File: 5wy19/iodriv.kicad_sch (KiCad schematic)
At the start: 17 parts, among them IC10 MC33385, IC3 74HCT574, IC4 HIP0045, IC6 MC33385, IC8 MC33385, Q7 BCR183

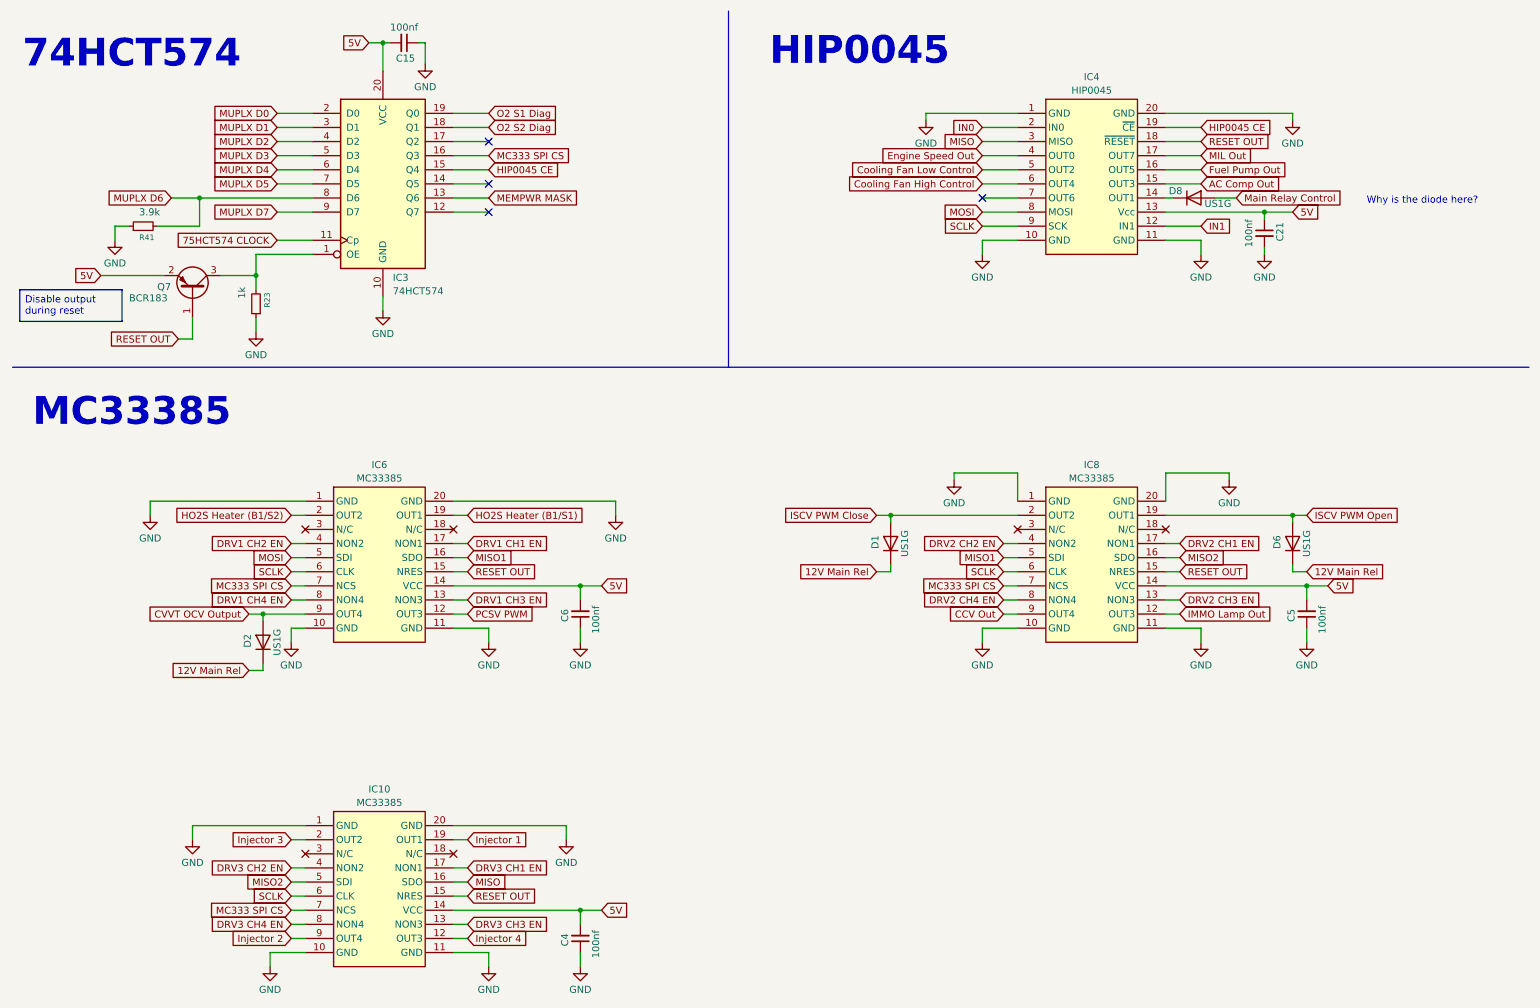
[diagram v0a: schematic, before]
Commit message: Final schematic (except maybe some oversights)
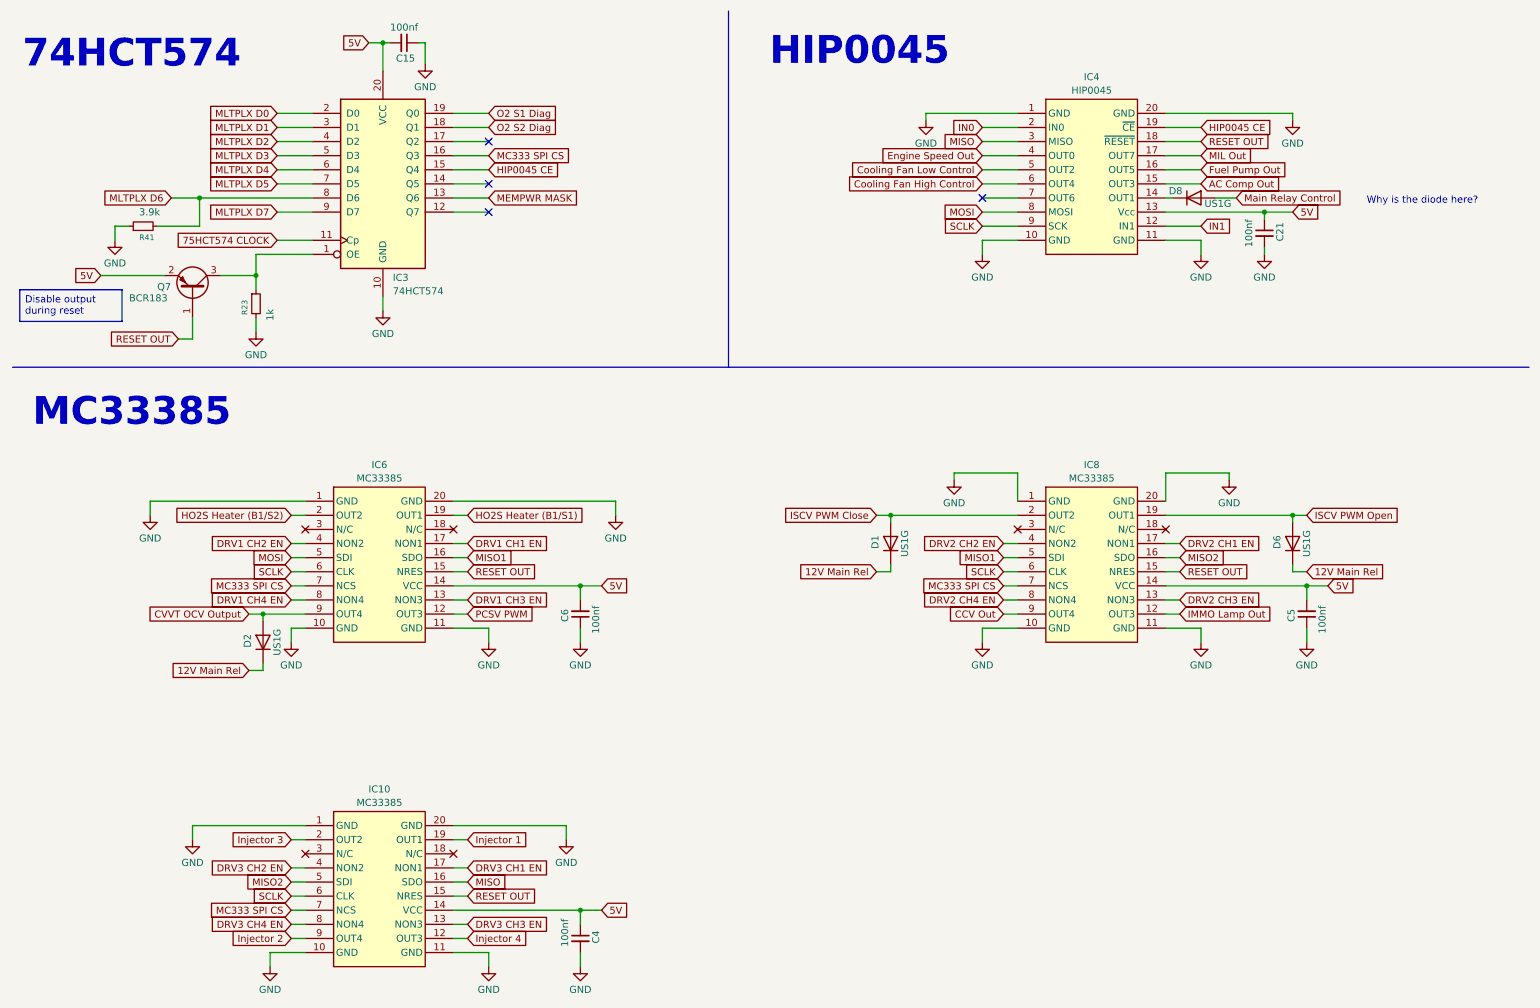
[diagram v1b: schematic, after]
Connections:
- net 5V: now also C4.1; no longer C4.2
- net GND: now also C4.2, R23.2; no longer C4.1, R23.1
- net at IC3.1 (OE), Q7.3 (C): now also R23.1; no longer R23.2
- net MUPLX D0 renamed MLTPLX D0
- net MUPLX D1 renamed MLTPLX D1
- net MUPLX D2 renamed MLTPLX D2
- net MUPLX D3 renamed MLTPLX D3
- net MUPLX D4 renamed MLTPLX D4
- net MUPLX D5 renamed MLTPLX D5
- net MUPLX D6 renamed MLTPLX D6
- net MUPLX D7 renamed MLTPLX D7
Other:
- moved on the sheet: C4, R23
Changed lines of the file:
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@@
 		)
 	)
-	(global_label "MUPLX D0"
-		(shape input)
-		(at 59.69 30.48 180)
-		(fields_autoplaced yes)
-		(effects
-			(font
-				(size 1.27 1.27)
-			)
-			(justify right)
-		)
-		(property "Intersheetrefs" "${INTERSHEET_REFS}"
-			(at 46.9682 30.48 0)
-			(effects
-				(font
-					(size 1.27 1.27)
-				)
-				(justify right)
-				(hide yes)
-			)
-		)
-	)
 	(global_label "Injector 4"
 		(shape input)
@@
 		)
 	)
-	(global_label "MUPLX D4"
-		(shape input)
-		(at 59.69 40.64 180)
-		(fields_autoplaced yes)
-		(effects
-			(font
-				(size 1.27 1.27)
-			)
-			(justify right)
-		)
-		(property "Intersheetrefs" "${INTERSHEET_REFS}"
-			(at 46.9682 40.64 0)
-			(effects
-				(font
-					(size 1.27 1.27)
-				)
-				(justify right)
-				(hide yes)
-			)
-		)
-	)
 	(global_label "DRV3 CH1 EN"
 		(shape input)
@@
 		)
 	)
-	(global_label "MUPLX D6"
+	(global_label "5V"
 		(shape input)
-		(at 40.64 45.72 180)
+		(at 27.94 59.69 180)
 		(fields_autoplaced yes)
 		(effects
@@
 		)
 		(property "Intersheetrefs" "${INTERSHEET_REFS}"
-			(at 27.9182 45.72 0)
+			(at 22.6567 59.69 0)
 			(effects
 				(font
@@
 		)
 	)
-	(global_label "5V"
+	(global_label "MLTPLX D5"
 		(shape input)
-		(at 27.94 59.69 180)
+		(at 59.69 43.18 180)
 		(fields_autoplaced yes)
 		(effects
@@
 		)
 		(property "Intersheetrefs" "${INTERSHEET_REFS}"
-			(at 22.6567 59.69 0)
+			(at 46.303 43.18 0)
 			(effects
 				(font
@@
 		)
 	)
+	(global_label "MLTPLX D7"
+		(shape input)
+		(at 59.69 48.26 180)
+		(fields_autoplaced yes)
+		(effects
+			(font
+				(size 1.27 1.27)
+			)
+			(justify right)
+		)
+		(property "Intersheetrefs" "${INTERSHEET_REFS}"
+			(at 46.303 48.26 0)
+			(effects
+				(font
+					(size 1.27 1.27)
+				)
+				(justify right)
+				(hide yes)
+			)
+		)
+	)
+	(global_label "MLTPLX D6"
+		(shape input)
+		(at 40.64 45.72 180)
+		(fields_autoplaced yes)
+		(effects
+			(font
+				(size 1.27 1.27)
+			)
+			(justify right)
+		)
+		(property "Intersheetrefs" "${INTERSHEET_REFS}"
+			(at 27.253 45.72 0)
+			(effects
+				(font
+					(size 1.27 1.27)
+				)
+				(justify right)
+				(hide yes)
+			)
+		)
+	)
 	(global_label "12V Main Rel"
 		(shape input)
@@
 		)
 	)
-	(global_label "MUPLX D1"
-		(shape input)
-		(at 59.69 33.02 180)
-		(fields_autoplaced yes)
-		(effects
-			(font
-				(size 1.27 1.27)
-			)
-			(justify right)
-		)
-		(property "Intersheetrefs" "${INTERSHEET_REFS}"
-			(at 46.9682 33.02 0)
-			(effects
-				(font
-					(size 1.27 1.27)
-				)
-				(justify right)
-				(hide yes)
-			)
-		)
-	)
 	(global_label "5V"
 		(shape input)
@@
 		)
 	)
-	(global_label "MUPLX D3"
+	(global_label "MLTPLX D2"
 		(shape input)
-		(at 59.69 38.1 180)
+		(at 59.69 35.56 180)
 		(fields_autoplaced yes)
 		(effects
@@
 		)
 		(property "Intersheetrefs" "${INTERSHEET_REFS}"
-			(at 46.9682 38.1 0)
+			(at 46.303 35.56 0)
 			(effects
 				(font
@@
 		)
 	)
+	(global_label "MLTPLX D3"
+		(shape input)
+		(at 59.69 38.1 180)
+		(fields_autoplaced yes)
+		(effects
+			(font
+				(size 1.27 1.27)
+			)
+			(justify right)
+		)
+		(property "Intersheetrefs" "${INTERSHEET_REFS}"
+			(at 46.303 38.1 0)
+			(effects
+				(font
+					(size 1.27 1.27)
+				)
+				(justify right)
+				(hide yes)
+			)
+		)
+	)
 	(global_label "MISO2"
 		(shape input)
@@
 		)
 	)
-	(global_label "DRV2 CH1 EN"
+	(global_label "MLTPLX D1"
 		(shape input)
-		(at 222.25 107.95 0)
+		(at 59.69 33.02 180)
 		(fields_autoplaced yes)
 		(effects
@@
 				(size 1.27 1.27)
 			)
-			(justify left)
+			(justify right)
 		)
 		(property "Intersheetrefs" "${INTERSHEET_REFS}"
-			(at 238.298 107.95 0)
+			(at 46.303 33.02 0)
 			(effects
 				(font
 					(size 1.27 1.27)
 				)
-				(justify left)
+				(justify right)
 				(hide yes)
 			)
 		)
 	)
-	(global_label "DRV2 CH3 EN"
+	(global_label "DRV2 CH1 EN"
 		(shape input)
-		(at 222.25 118.11 0)
+		(at 222.25 107.95 0)
 		(fields_autoplaced yes)
 		(effects
@@
 		)
 		(property "Intersheetrefs" "${INTERSHEET_REFS}"
-			(at 238.298 118.11 0)
+			(at 238.298 107.95 0)
 			(effects
 				(font
@@
 		)
 	)
-	(global_label "MUPLX D7"
+	(global_label "DRV2 CH3 EN"
 		(shape input)
-		(at 59.69 48.26 180)
+		(at 222.25 118.11 0)
 		(fields_autoplaced yes)
 		(effects
@@
 				(size 1.27 1.27)
 			)
-			(justify right)
+			(justify left)
 		)
 		(property "Intersheetrefs" "${INTERSHEET_REFS}"
-			(at 46.9682 48.26 0)
+			(at 238.298 118.11 0)
 			(effects
 				(font
 					(size 1.27 1.27)
 				)
-				(justify right)
+				(justify left)
 				(hide yes)
 			)
@@
 		)
 	)
-	(global_label "MUPLX D5"
+	(global_label "MIL Out"
 		(shape input)
-		(at 59.69 43.18 180)
+		(at 226.06 38.1 0)
 		(fields_autoplaced yes)
 		(effects
@@
 				(size 1.27 1.27)
 			)
-			(justify right)
+			(justify left)
 		)
 		(property "Intersheetrefs" "${INTERSHEET_REFS}"
-			(at 46.9682 43.18 0)
+			(at 236.3023 38.1 0)
 			(effects
 				(font
 					(size 1.27 1.27)
 				)
-				(justify right)
+				(justify left)
 				(hide yes)
 			)
 		)
 	)
-	(global_label "MIL Out"
+	(global_label "SCLK"
 		(shape input)
-		(at 226.06 38.1 0)
+		(at 62.23 113.03 180)
 		(fields_autoplaced yes)
 		(effects
@@
 				(size 1.27 1.27)
 			)
-			(justify left)
+			(justify right)
 		)
 		(property "Intersheetrefs" "${INTERSHEET_REFS}"
-			(at 236.3023 38.1 0)
+			(at 54.4672 113.03 0)
 			(effects
 				(font
 					(size 1.27 1.27)
 				)
-				(justify left)
+				(justify right)
 				(hide yes)
 			)
 		)
 	)
-	(global_label "SCLK"
+	(global_label "Injector 3"
 		(shape input)
-		(at 62.23 113.03 180)
+		(at 62.23 161.29 180)
 		(fields_autoplaced yes)
 		(effects
@@
 		)
 		(property "Intersheetrefs" "${INTERSHEET_REFS}"
-			(at 54.4672 113.03 0)
+			(at 49.871 161.29 0)
 			(effects
 				(font
@@
 		)
 	)
-	(global_label "MUPLX D2"
+	(global_label "MLTPLX D0"
 		(shape input)
-		(at 59.69 35.56 180)
+		(at 59.69 30.48 180)
 		(fields_autoplaced yes)
 		(effects
@@
 		)
 		(property "Intersheetrefs" "${INTERSHEET_REFS}"
-			(at 46.9682 35.56 0)
+			(at 46.303 30.48 0)
 			(effects
 				(font
@@
 		)
 	)
-	(global_label "Injector 3"
+	(global_label "MISO2"
 		(shape input)
-		(at 62.23 161.29 180)
+		(at 222.25 110.49 0)
 		(fields_autoplaced yes)
 		(effects
@@
 				(size 1.27 1.27)
 			)
-			(justify right)
+			(justify left)
 		)
 		(property "Intersheetrefs" "${INTERSHEET_REFS}"
-			(at 49.871 161.29 0)
+			(at 231.0409 110.49 0)
 			(effects
 				(font
 					(size 1.27 1.27)
 				)
-				(justify right)
+				(justify left)
 				(hide yes)
 			)
 		)
 	)
-	(global_label "MISO2"
+	(global_label "MLTPLX D4"
 		(shape input)
-		(at 222.25 110.49 0)
+		(at 59.69 40.64 180)
 		(fields_autoplaced yes)
 		(effects
@@
 				(size 1.27 1.27)
 			)
-			(justify left)
+			(justify right)
 		)
 		(property "Intersheetrefs" "${INTERSHEET_REFS}"
-			(at 231.0409 110.49 0)
+			(at 46.303 40.64 0)
 			(effects
 				(font
 					(size 1.27 1.27)
 				)
-				(justify left)
+				(justify right)
 				(hide yes)
 			)
@@
 	(symbol
 		(lib_id "Device:C_Small")
-		(at 114.3 179.07 180)
+		(at 114.3 179.07 0)
 		(unit 1)
 		(exclude_from_sim no)
@@
 		(dnp no)
 		(property "Reference" "C4"
-			(at 111.506 179.324 90)
+			(at 117.094 178.816 90)
 			(effects
 				(font
@@
 		)
 		(property "Value" "100nf"
-			(at 117.094 180.086 90)
+			(at 111.506 178.054 90)
 			(effects
 				(font
@@
 	(symbol
 		(lib_id "Device:R_Small")
-		(at 55.88 64.77 180)
+		(at 55.88 64.77 0)
 		(unit 1)
 		(exclude_from_sim no)
@@
 		(dnp no)
 		(property "Reference" "R23"
-			(at 57.912 62.738 90)
+			(at 53.848 66.802 90)
 			(effects
 				(font
@@
 		)
 		(property "Value" "1k"
-			(at 53.34 61.722 90)
+			(at 58.42 67.818 90)
 			(effects
 				(font
